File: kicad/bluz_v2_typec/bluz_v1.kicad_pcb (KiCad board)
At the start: 2 copper layers, 29.6 x 16.1 mm, 76 parts, among them J10 Conn, J11 Conn, J12 BTAnt, J2 Conn, J3 Conn, J4 Conn, J5 Conn, J6 Conn, J7 Conn, J8 Conn, J9 USB_C_Receptacle_PowerOnly_6P, M1 Z3OC1T8219731, Q2 RUM002N05, SW1 SW_DPDT_x2, U1 MCP73831, U3 TLV3201AIDCK, U4 AP3015KTR, U5 MCP1700-1.8, U6 PAM8904EGPR, U7 TPS627451DSSR, Y1 NX1612SA-32MHz, Y2 NX2012SA-32.768

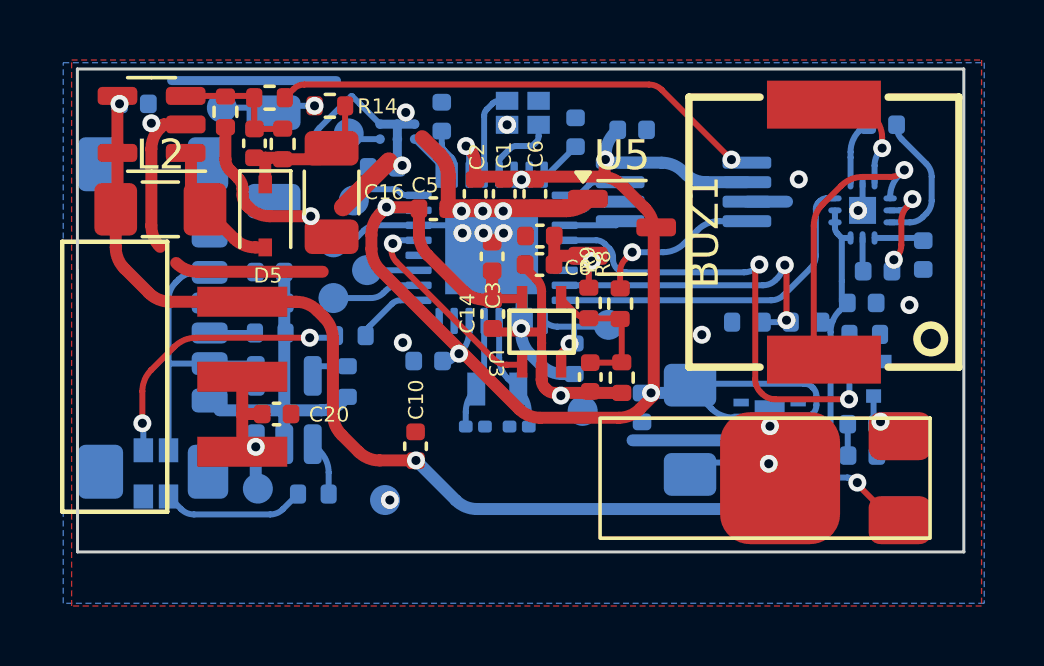
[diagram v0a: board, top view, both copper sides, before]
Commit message: изменено:      kicad/bluz_v2_typec/bluz_v1.kicad_pcb
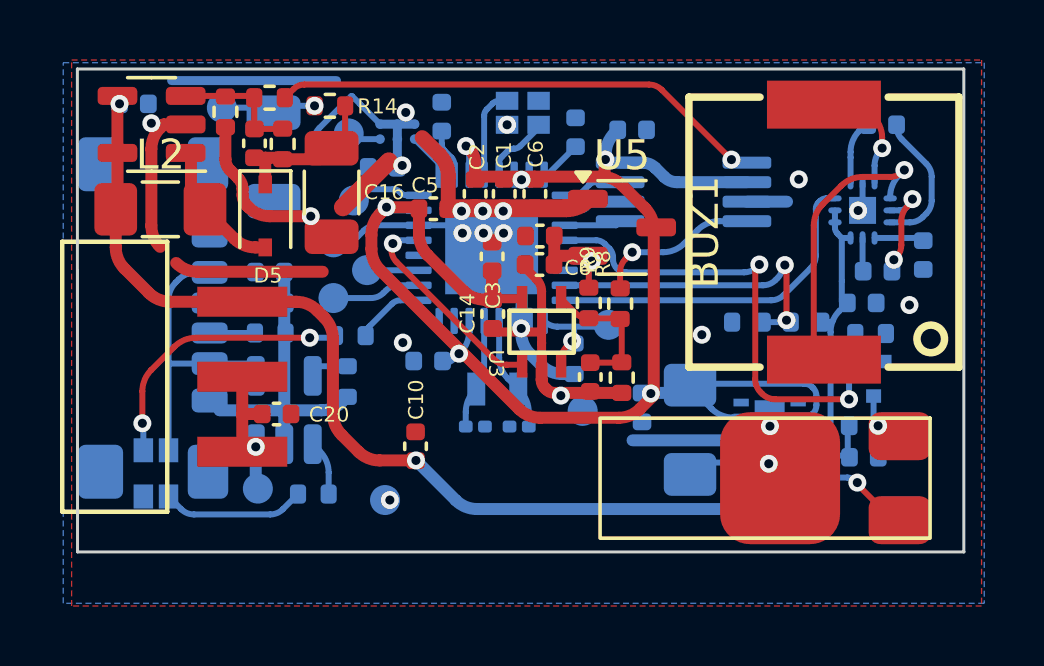
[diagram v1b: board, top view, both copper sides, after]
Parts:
- moved R12 0.20 mm to (119.9, 54.4)
- moved C24 0.07 mm to (119.7, 58.5)
- moved C26 0.07 mm to (119.6, 57.4)
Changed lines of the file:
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@@
 	(footprint "Capacitor_SMD:C_0402_1005Metric"
 		(layer "B.Cu")
-		(at 119.602086 58.417741 180)
+		(at 119.65 58.475 180)
 		(descr "Capacitor SMD 0402 (1005 Metric), square (rectangular) end terminal, IPC_7351 nominal, (Body size source: IPC-SM-782 page 76, https://www.pcb-3d.com/wordpress/wp-content/uploads/ipc-sm-782a_amendment_1_and_2.pdf), generated with kicad-footprint-generator")
 		(tags "capacitor")
@@
 	(footprint "Capacitor_SMD:C_0402_1005Metric"
 		(layer "B.Cu")
-		(at 119.59266 57.371456)
+		(at 119.640574 57.428715)
 		(descr "Capacitor SMD 0402 (1005 Metric), square (rectangular) end terminal, IPC-7351 nominal, (Body size source: IPC-SM-782 page 76, https://www.pcb-3d.com/wordpress/wp-content/uploads/ipc-sm-782a_amendment_1_and_2.pdf), generated with kicad-footprint-generator")
 		(tags "capacitor")
@@
 	(footprint "Resistor_SMD:R_0402_1005Metric"
 		(layer "B.Cu")
-		(at 119.679977 54.379031)
+		(at 119.875 54.35)
 		(descr "Resistor SMD 0402 (1005 Metric), square (rectangular) end terminal, IPC_7351 nominal, (Body size source: IPC-SM-782 page 72, https://www.pcb-3d.com/wordpress/wp-content/uploads/ipc-sm-782a_amendment_1_and_2.pdf), generated with kicad-footprint-generator")
 		(tags "resistor")
@@
 	)
 	(via
-		(at 112.557246 56.330621)
+		(at 112.55 56.35)
 		(size 0.6)
 		(drill 0.3)
@@
 	)
 	(segment
-		(start 106.493128 53.92976)
-		(end 106.493128 54.282658)
-		(width 0.2)
+		(start 115.7525 49.305)
+		(end 113.423528 49.305)
+		(width 0.4)
 		(layer "B.Cu")
 		(net 2)
 	)
 	(segment
-		(start 106.493128 49.05476)
-		(end 106.493128 48.303128)
-		(width 0.2)
+		(start 112.999264 49.129264)
+		(end 112.700736 48.830736)
+		(width 0.4)
 		(layer "B.Cu")
 		(net 2)
 	)
 	(segment
-		(start 104.805628 50.24226)
-		(end 103.84226 50.24226)
+		(start 106.493128 53.92976)
+		(end 106.493128 54.282658)
 		(width 0.2)
 		(layer "B.Cu")
@@
 	)
 	(segment
-		(start 114.389214 49.305)
-		(end 115.7525 49.305)
-		(width 0.4)
+		(start 106.493128 49.05476)
+		(end 106.493128 48.303128)
+		(width 0.2)
 		(layer "B.Cu")
 		(net 2)
 	)
 	(segment
-		(start 111.5275 48.655)
-		(end 112.910786 48.655)
-		(width 0.4)
+		(start 104.805628 50.24226)
+		(end 103.84226 50.24226)
+		(width 0.2)
 		(layer "B.Cu")
 		(net 2)
@@
 	)
 	(segment
+		(start 112.276472 48.655)
+		(end 111.5275 48.655)
+		(width 0.4)
+		(layer "B.Cu")
+		(net 2)
+	)
+	(segment
 		(start 117.952842 56.155842)
 		(end 117.93744 56.14044)
@@
 	)
 	(segment
-		(start 113.617893 48.947893)
-		(end 113.682107 49.012107)
-		(width 0.2)
-		(layer "B.Cu")
-		(net 2)
-	)
-	(segment
 		(start 117.937157 57.032843)
 		(end 117.952842 57.017158)
@@
 	)
 	(arc
-		(start 114.389214 49.305)
-		(mid 114.006531 49.22888)
-		(end 113.682107 49.012107)
-		(width 0.4)
-		(layer "B.Cu")
-		(net 2)
-	)
-	(arc
 		(start 106.493128 54.282658)
 		(mid 106.417008 54.665341)
@@
 	)
 	(arc
-		(start 112.910786 48.655)
-		(mid 113.293469 48.73112)
-		(end 113.617893 48.947893)
-		(width 0.4)
-		(layer "B.Cu")
-		(net 2)
-	)
-	(arc
 		(start 105.571472 55.36)
 		(mid 105.801082 55.314328)
@@
 	)
 	(arc
+		(start 112.999264 49.129264)
+		(mid 113.193918 49.259328)
+		(end 113.423528 49.305)
+		(width 0.4)
+		(layer "B.Cu")
+		(net 2)
+	)
+	(arc
+		(start 112.700736 48.830736)
+		(mid 112.506082 48.700672)
+		(end 112.276472 48.655)
+		(width 0.4)
+		(layer "B.Cu")
+		(net 2)
+	)
+	(arc
 		(start 117.93744 56.14044)
 		(mid 117.807671 56.053731)
@@
 	)
 	(segment
-		(start 109.56 54.97)
+		(start 109.735736 54.794264)
 		(end 109.84 54.69)
 		(width 0.2)
@@
 	(segment
 		(start 109.56 55.39)
-		(end 109.56 54.97)
+		(end 109.56 55.218528)
 		(width 0.2)
 		(layer "F.Cu")
@@
 	)
 	(via
-		(at 109.84 54.69)
+		(at 109.925 54.6)
 		(size 0.6)
 		(drill 0.3)
@@
 		(net 9)
 	)
+	(arc
+		(start 109.735736 54.794264)
+		(mid 109.605672 54.988918)
+		(end 109.56 55.218528)
+		(width 0.2)
+		(layer "F.Cu")
+		(net 9)
+	)
 	(segment
 		(start 109.99 54.12)
@@
 	)
 	(segment
-		(start 116.08285 52.134264)
-		(end 116.167114 52.05)
+		(start 119.332047 55.525879)
+		(end 119.574539 55.283387)
 		(width 0.2)
 		(layer "B.Cu")
@@
 	)
 	(segment
-		(start 109.680628 51.24226)
-		(end 110.726575 51.24226)
+		(start 116.08285 52.134264)
+		(end 116.167114 52.05)
 		(width 0.2)
 		(layer "B.Cu")
@@
 	)
 	(segment
-		(start 119.184034 55.283387)
-		(end 119.169977 55.26933)
+		(start 109.680628 51.24226)
+		(end 110.726575 51.24226)
 		(width 0.2)
 		(layer "B.Cu")
@@
 	)
 	(segment
-		(start 111.29 51.805685)
-		(end 111.29 51.884315)
+		(start 119.574539 55.283387)
+		(end 119.574539 54.808067)
 		(width 0.2)
 		(layer "B.Cu")
@@
 	)
 	(segment
-		(start 119.574539 55.283387)
-		(end 119.184034 55.283387)
+		(start 111.29 51.805685)
+		(end 111.29 51.884315)
 		(width 0.2)
 		(layer "B.Cu")
@@
 	)
 	(segment
-		(start 119.169977 56.52732)
-		(end 119.169977 55.26933)
+		(start 119.156311 56.540986)
+		(end 119.156311 55.950143)
 		(width 0.2)
 		(layer "B.Cu")
@@
 	)
 	(segment
-		(start 119.169977 55.26933)
-		(end 119.169977 54.379031)
+		(start 111.715685 52.31)
+		(end 115.658586 52.31)
 		(width 0.2)
 		(layer "B.Cu")
@@
 	)
 	(segment
-		(start 111.715685 52.31)
-		(end 115.658586 52.31)
+		(start 119.156311 56.540986)
+		(end 119.169977 56.52732)
 		(width 0.2)
 		(layer "B.Cu")
@@
 	)
 	(segment
-		(start 119.156311 56.540986)
-		(end 119.169977 56.52732)
+		(start 119.398803 54.383803)
+		(end 119.365 54.35)
 		(width 0.2)
 		(layer "B.Cu")
@@
 	)
 	(arc
+		(start 119.156311 55.950143)
+		(mid 119.201983 55.720533)
+		(end 119.332047 55.525879)
+		(width 0.2)
+		(layer "B.Cu")
+		(net 10)
+	)
+	(arc
+		(start 119.574539 54.808067)
+		(mid 119.528867 54.578457)
+		(end 119.398803 54.383803)
+		(width 0.2)
+		(layer "B.Cu")
+		(net 10)
+	)
+	(arc
 		(start 111.172843 51.522843)
 		(mid 111.259552 51.652612)
@@
 	)
 	(segment
-		(start 108.688256 48.012132)
-		(end 108.72026 47.980128)
+		(start 107.976396 48.187868)
+		(end 107.987868 48.187868)
 		(width 0.2)
 		(layer "B.Cu")
@@
 	)
 	(segment
-		(start 108.808128 47.767996)
-		(end 108.808128 47.39226)
+		(start 108.2 48.1)
+		(end 108.75 47.55)
 		(width 0.2)
 		(layer "B.Cu")
@@
 	(segment
 		(start 107.580996 48.459004)
-		(end 107.852132 48.187868)
-		(width 0.2)
-		(layer "B.Cu")
-		(net 24)
-	)
-	(segment
-		(start 108.064264 48.1)
-		(end 108.476124 48.1)
+		(end 107.764264 48.275736)
 		(width 0.2)
 		(layer "B.Cu")
@@
 	)
 	(arc
-		(start 108.808128 47.767996)
-		(mid 108.785292 47.882801)
-		(end 108.72026 47.980128)
-		(width 0.2)
-		(layer "B.Cu")
-		(net 24)
-	)
-	(arc
-		(start 108.476124 48.1)
-		(mid 108.590929 48.077164)
-		(end 108.688256 48.012132)
+		(start 107.764264 48.275736)
+		(mid 107.861591 48.210704)
+		(end 107.976396 48.187868)
 		(width 0.2)
 		(layer "B.Cu")
@@
 	)
 	(arc
-		(start 107.852132 48.187868)
-		(mid 107.949459 48.122836)
-		(end 108.064264 48.1)
+		(start 107.987868 48.187868)
+		(mid 108.102673 48.165032)
+		(end 108.2 48.1)
 		(width 0.2)
 		(layer "B.Cu")
@@
 	)
 	(segment
-		(start 120.210197 58.340449)
-		(end 120.287489 58.417741)
-		(width 0.2)
-		(layer "B.Cu")
-		(net 26)
-	)
-	(segment
 		(start 108.493128 53.92976)
 		(end 107.993128 53.92976)
@@
 	)
 	(via
-		(at 120.205349 57.28809)
+		(at 120.125 57.425)
 		(size 0.6)
 		(drill 0.3)

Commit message: изменено:      kicad/bluz_v2_typec/bluz_v1.kicad_pcb 	изменено:      kicad/bluz_v2_typec/bluz_v1.kicad_sch
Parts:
- R1: value 510k -> 1.3M
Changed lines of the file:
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@@
 			)
 		)
-		(property "Value" "510k"
+		(property "Value" "1.3M"
 			(at 0 -1.17 0)
 			(layer "B.Fab")
